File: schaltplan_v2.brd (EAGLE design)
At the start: 100 x 80 mm, 9 parts, among them T1 2N3565, T2 2N3565, X1 SSW-102-02-S-S-RA, X3 SSW-103-02-S-S-RA, X4 SSW-109-02-S-S-RA

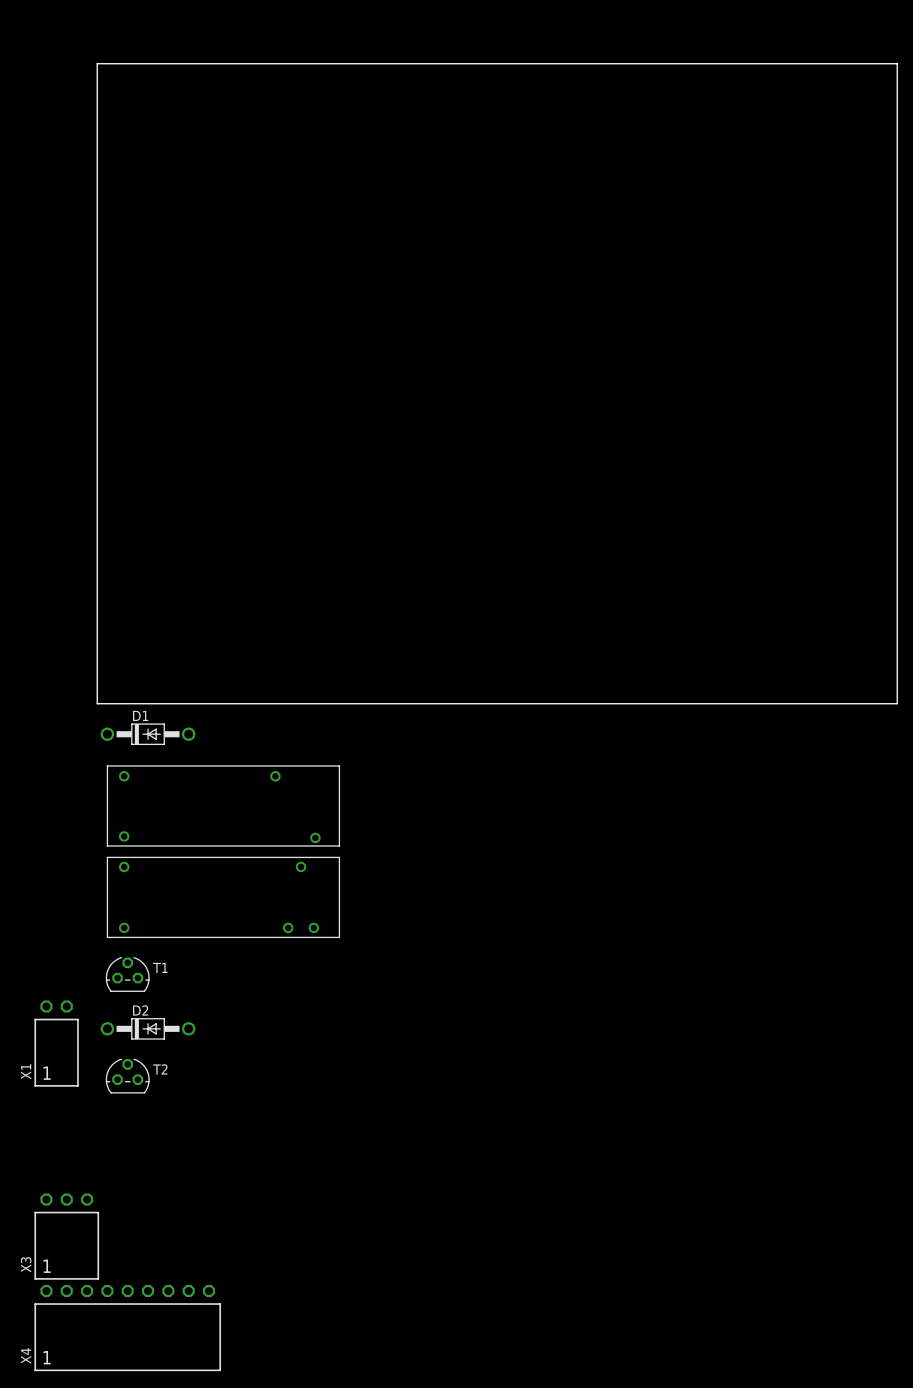
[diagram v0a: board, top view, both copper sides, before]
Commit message: schaltplan_v2 finalized
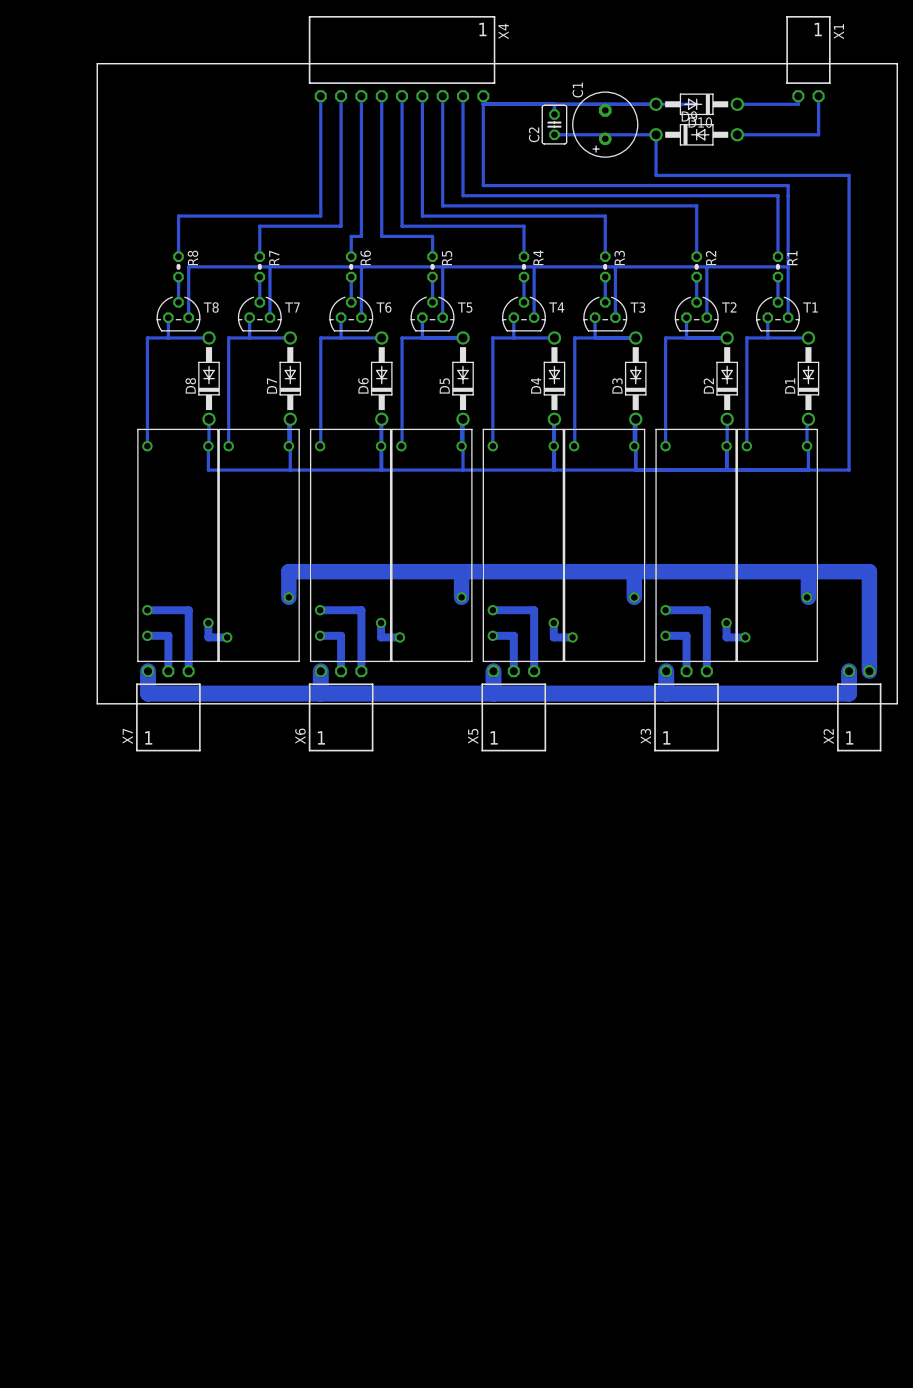
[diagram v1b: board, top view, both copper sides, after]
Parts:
- added C1: (no value), rcl:E3,5-8
- added C2: (no value), rcl:C025-030X050
- added D10, D3, D4, D5, D6, D7, D8, D9: 1N4004, diode:DO41-10
- added R1, R2, R3, R4, R5, R6, R7, R8: (no value), resistor:0204V
- added T3, T4, T5, T6, T7, T8: 2N3565, transistor:TO92
- added U$3, U$5, U$7: JS_05_MN_KT, n39:JS_05_MN_KT
- added U$4, U$6, U$8: JS_05_N_K, n39:JS_05_N_K
- added X2: SSW-102-02-S-S-RA, con-samtec:SSW-102-02-S-S-RA
- added X5, X6, X7: SSW-103-02-S-S-RA, con-samtec:SSW-103-02-S-S-RA
- moved X4 156.2 mm to (38.1, 77.5), turned to 180 degrees
- moved X1 149.9 mm to (88.9, 77.5), turned to 180 degrees
- moved T2 118.9 mm to (74.9, 48.3)
- moved T1 115.8 mm to (85.1, 48.3)
- moved D2 108.8 mm to (78.7, 40.6), turned to 90 degrees
- moved X3 101.8 mm to (73.7, 2.54)
- moved U$1 94.4 mm to (80.0, 34.3), turned to 270 degrees
- moved D1 93.8 mm to (88.9, 40.6), turned to 90 degrees
- moved U$2 93.5 mm to (69.8, 34.3), turned to 270 degrees
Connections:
- new net N$1: X2.1, X3.1, X5.1, X6.1, X7.1
- new net N$10: C1.-, C2.2, D10.A, T1.1, T2.1, T3.1, T4.1, T5.1, T6.1, T7.1, T8.1, X4.1
- new net N$11: R2.1, X4.3
- new net N$12: D2.A, T2.3, U$2.P$1
- new net N$13: R6.2, T6.2
- new net N$14: R3.1, X4.4
- new net N$16: U$4.P$5, X5.2
- new net N$17: U$4.P$4, X5.3
- new net N$18: U$3.P$4, U$4.P$3
- new net N$2: U$2.P$5, X3.2
- new net N$20: D3.A, T3.3, U$3.P$1
- new net N$21: C1.+, C2.1, D1.C, D2.C, D3.C, D4.C, D5.C, D6.C, D7.C, D8.C, D9.C, U$1.P$2, U$2.P$2, U$3.P$2, U$4.P$2, U$5.P$2, U$6.P$2, U$7.P$2, U$8.P$2
- new net N$22: R3.2, T3.2
- new net N$23: R4.1, X4.5
- new net N$25: D4.A, T4.3, U$4.P$1
- new net N$26: R5.1, X4.6
- new net N$27: R2.2, T2.2
- new net N$28: R4.2, T4.2
- new net N$3: U$2.P$4, X3.3
- new net N$30: U$6.P$5, X6.2
- new net N$31: U$6.P$4, X6.3
- new net N$32: U$5.P$4, U$6.P$3
- new net N$34: D5.A, T5.3, U$5.P$1
- new net N$36: R5.2, T5.2
- new net N$37: R6.1, X4.7
- new net N$39: D6.A, T6.3, U$6.P$1
- new net N$4: U$1.P$4, U$2.P$3
- new net N$40: R8.2, T8.2
- new net N$42: U$8.P$5, X7.2
- new net N$43: U$8.P$4, X7.3
- new net N$44: U$7.P$4, U$8.P$3
- new net N$46: D7.A, T7.3, U$7.P$1
- new net N$48: R7.2, T7.2
- new net N$49: R7.1, X4.8
- new net N$5: U$1.P$3, U$3.P$3, U$5.P$3, U$7.P$3, X2.2
- new net N$51: D8.A, T8.3, U$8.P$1
- new net N$53: D9.A, X1.1
- new net N$54: D10.C, X1.2
- new net N$6: D1.A, T1.3, U$1.P$1
- new net N$7: R8.1, X4.9
- new net N$8: R1.2, T1.2
- new net N$9: R1.1, X4.2
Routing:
- net N$21: track 0.00 -> 262.6 mm
- net N$10: track 0.00 -> 246.6 mm
- net N$1: track 0.00 -> 110.0 mm
- net N$5: track 0.00 -> 108.6 mm
- net N$9: track 0.00 -> 59.4 mm
- net N$11: track 0.00 -> 51.8 mm
- net N$14: track 0.00 -> 42.9 mm
- net N$7: track 0.00 -> 37.8 mm
- net N$23: track 0.00 -> 35.3 mm
- net N$49: track 0.00 -> 30.2 mm
- net N$20: track 0.00 -> 28.9 mm
- net N$34: track 0.00 -> 28.8 mm
- net N$12: track 0.00 -> 28.8 mm
- net N$26: track 0.00 -> 26.4 mm
- net N$6: track 0.00 -> 23.8 mm
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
